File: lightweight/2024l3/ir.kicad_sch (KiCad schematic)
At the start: 38 parts

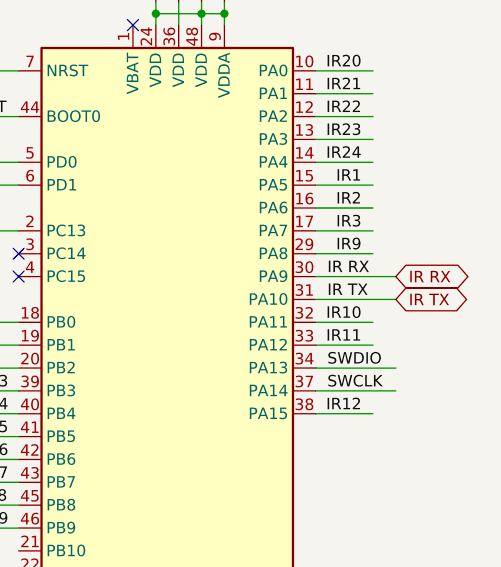
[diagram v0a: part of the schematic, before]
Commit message: lw - l3 - fixed serial
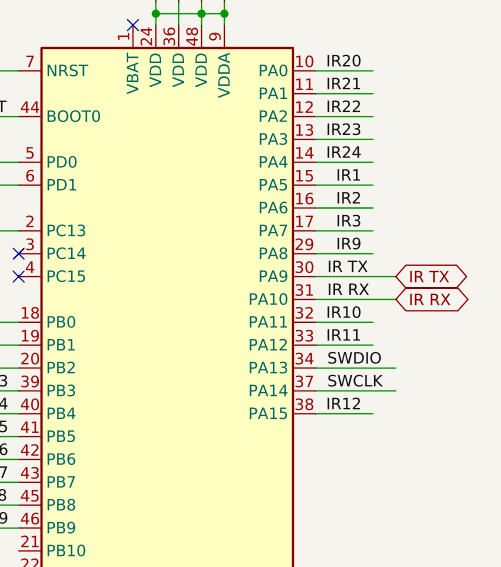
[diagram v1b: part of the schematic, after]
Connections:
- net IR RX: now also U?.31 (PA10); no longer U?.30 (PA9)
- net IR TX: now also U?.30 (PA9); no longer U?.31 (PA10)
